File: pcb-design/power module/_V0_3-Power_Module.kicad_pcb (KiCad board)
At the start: 2 copper layers, 76 x 56 mm, 18 parts, among them J16 SolarPowerIn and INA219, J17 CN3971, J18 TPS63020-GND-OUT, J19 TPS63020-V-IN, J20 ConnectorHiveScale, J21 MAXS17048, J23 TPS63020-3.3V-OUT, J6 TPS63020-GND-IN, m3-bl MountingHole_3.2mm_M3, m3-br MountingHole_3.2mm_M3, m3-tl MountingHole_3.2mm_M3, m3-tr MountingHole_3.2mm_M3

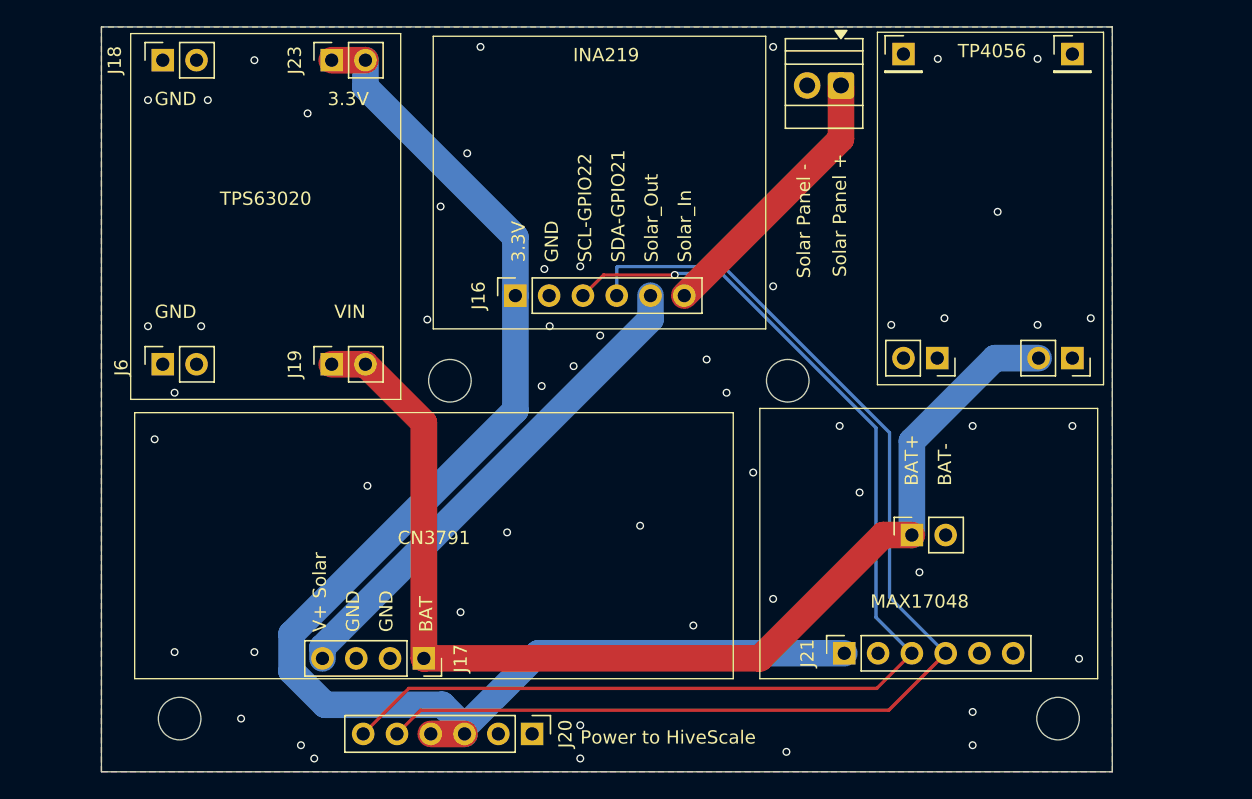
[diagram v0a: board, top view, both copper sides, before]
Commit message: updated pcb design
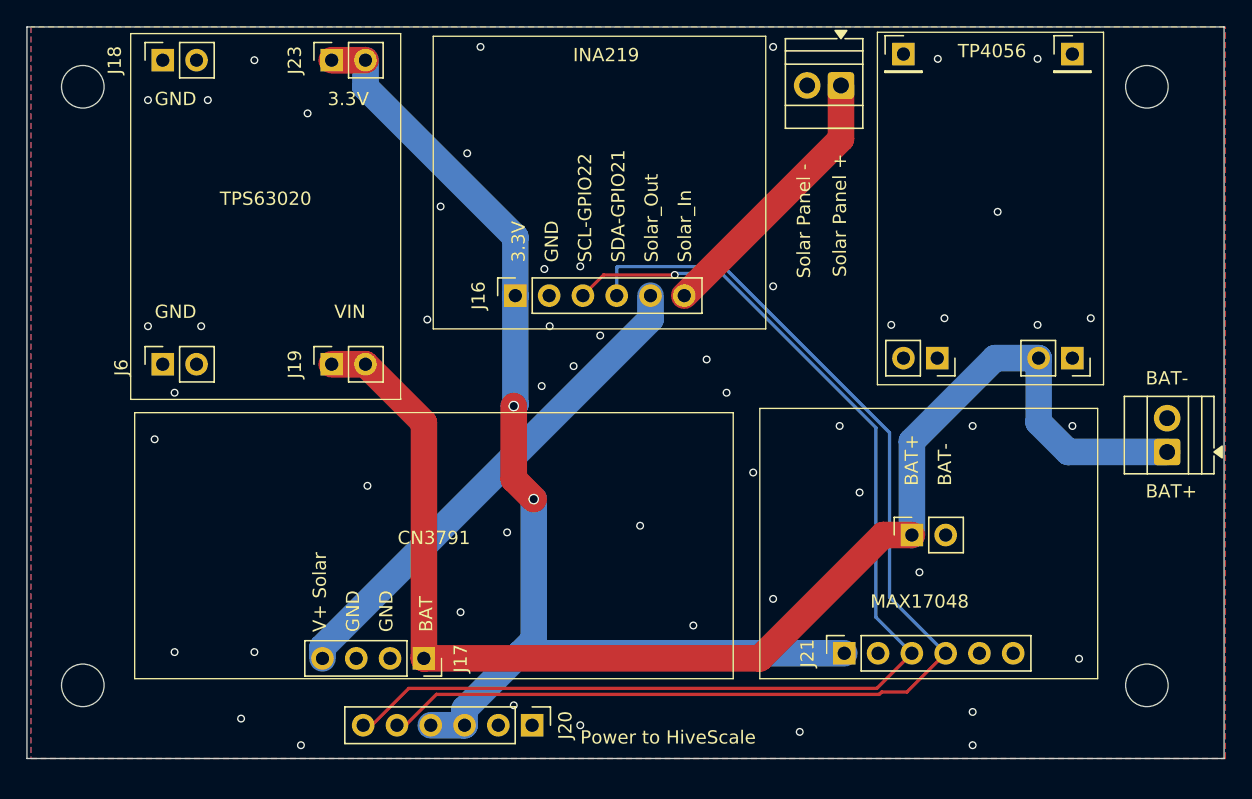
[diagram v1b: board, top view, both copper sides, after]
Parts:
- added Bat_Connector1: Battery, TerminalBlock:TerminalBlock_Xinya_XY308-2.54-2P_1x02_P2.54mm_Horizontal, F.Cu at (198.6, 74.0)
- moved m3-br 48.0 mm to (197.1, 46.5)
- moved m3-tr 35.4 mm to (197.1, 91.5)
- moved m3-tl 35.4 mm to (117.1, 46.5)
- moved m3-bl 7.70 mm to (117.1, 91.5)
- moved J20 0.65 mm to (150.9, 94.5)
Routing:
- net /3.3V: track 108.8 -> 86.9 mm, vias 0 -> 2
- net /BATpos: track 86.2 -> 101.6 mm
- net /BATneg: vias 52 -> 51
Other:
- board size 76 x 56 mm -> 90 x 55 mm
